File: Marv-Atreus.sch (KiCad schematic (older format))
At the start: 106 parts, among them SW1 SW_Push, U1 ATmega32U4-AU, Y1 16MHz

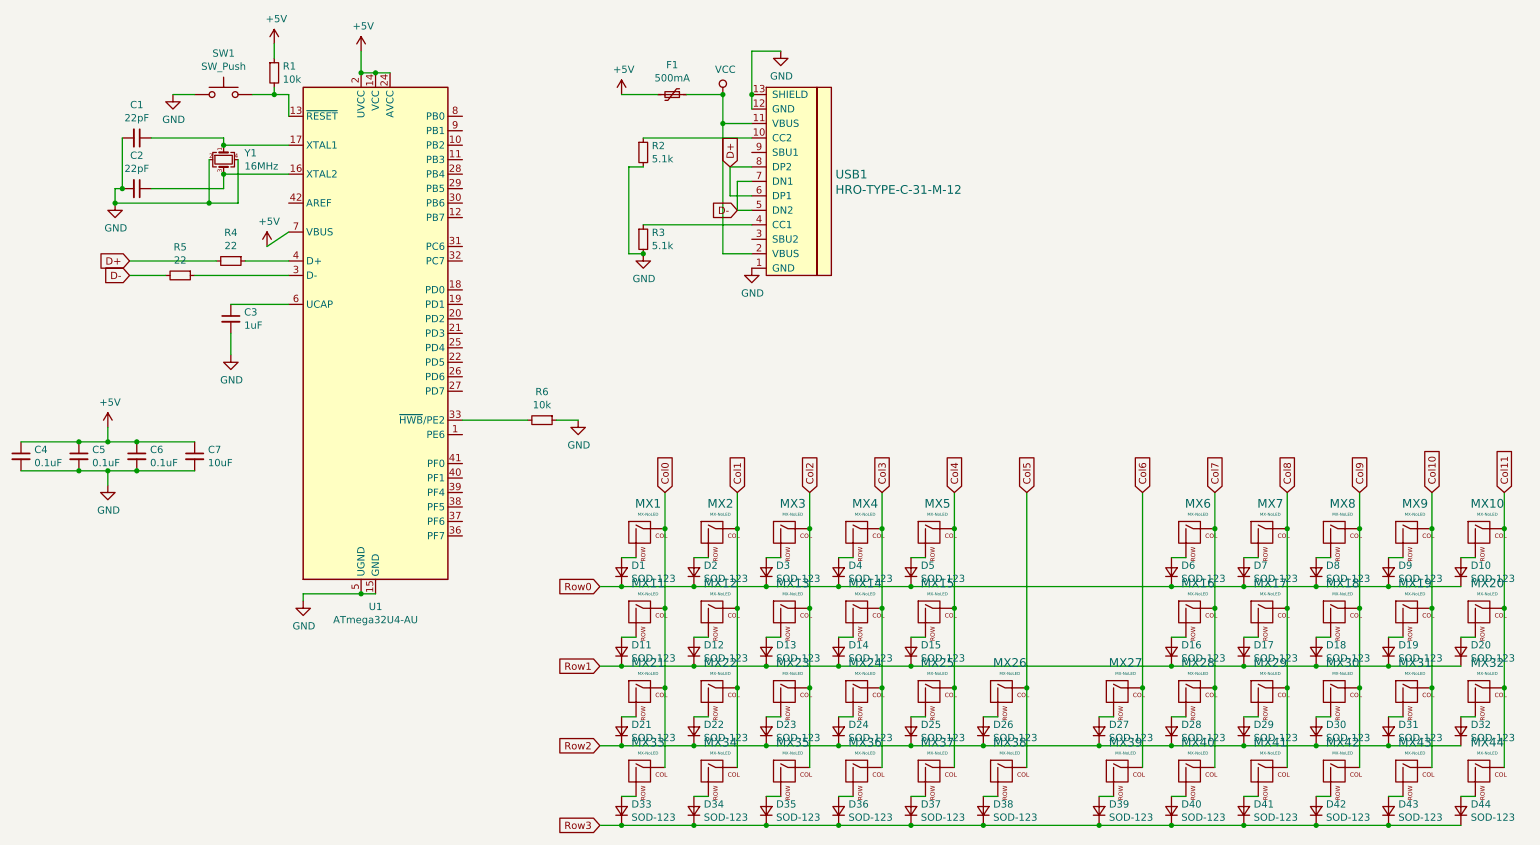
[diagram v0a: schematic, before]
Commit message: First Proto
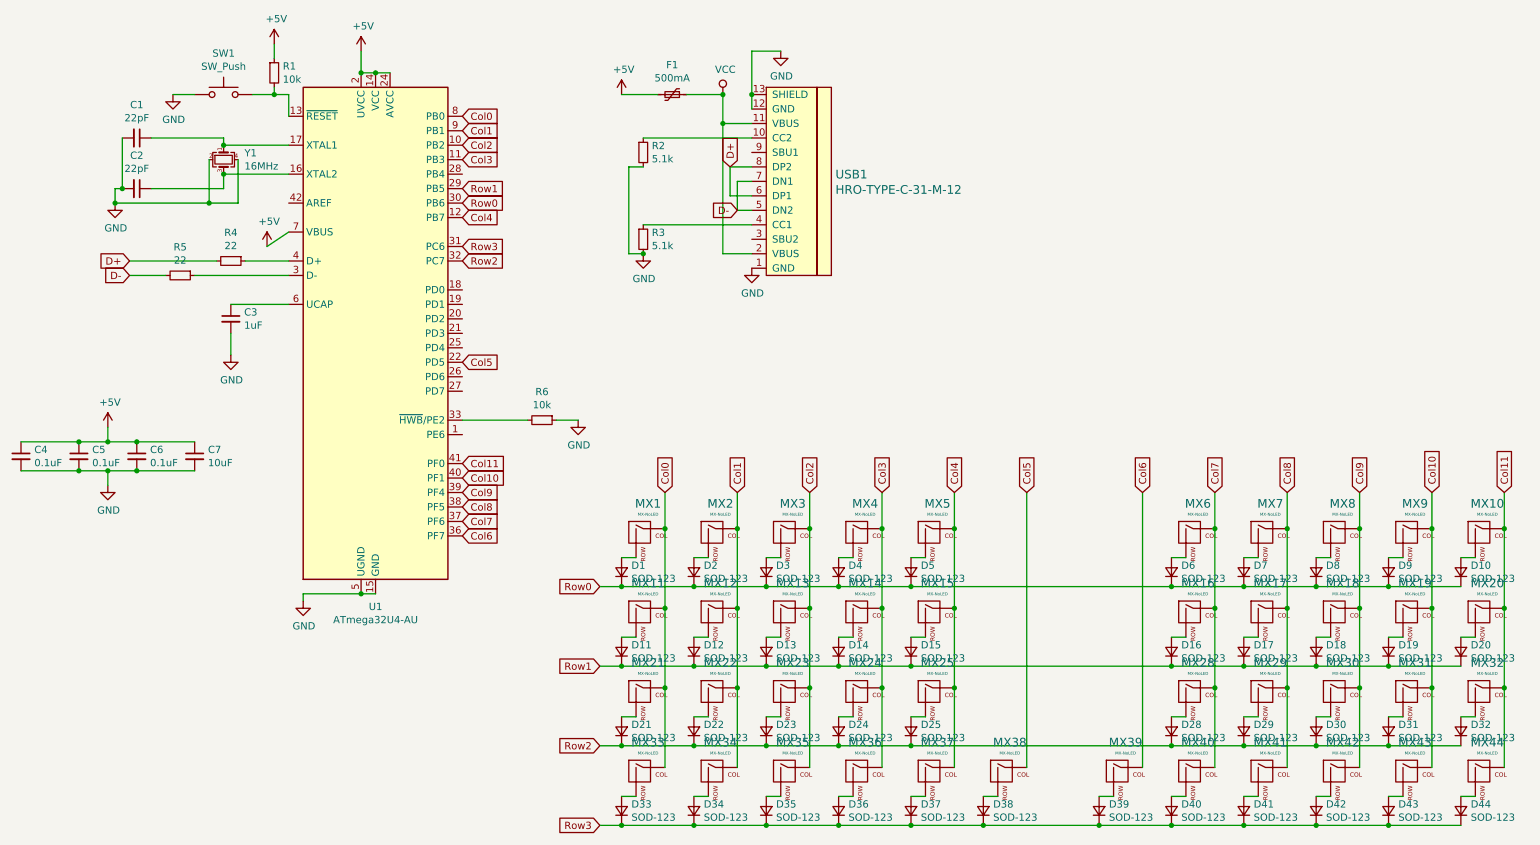
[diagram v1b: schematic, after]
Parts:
- removed D26, D27: SOD-123, Diode_SMD:D_SOD-123, symbol Device:D_Small
- removed MX26, MX27: MX-NoLED, MX_Only:MXOnly-1U-NoLED, symbol MX_Alps_Hybrid:MX-NoLED
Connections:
- net Col0: now also U1.8 (PB0)
- net Col1: now also U1.9 (PB1)
- net Col10: now also U1.40 (PF1)
- net Col11: now also U1.41 (PF0)
- net Col2: now also U1.10 (PB2)
- net Col3: now also U1.11 (PB3)
- net Col4: now also U1.12 (PB7)
- net Col5: now also U1.22 (PD5)
- net Col6: now also U1.36 (PF7)
- net Col7: now also U1.37 (PF6)
- net Col8: now also U1.38 (PF5)
- net Col9: now also U1.39 (PF4)
- net Row0: now also U1.30 (PB6)
- net Row1: now also U1.29 (PB5)
- net Row2: now also U1.32 (PC7)
- net Row3: now also U1.31 (PC6)
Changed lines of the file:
@@
 	6750 5900 6850 5900
-$Comp
-L MX_Alps_Hybrid:MX-NoLED MX26
-U 1 1 5EA47DBA
-P 7400 5200
-F 0 "MX26" H 7433 5423 60  0000 C CNN
-F 1 "MX-NoLED" H 7433 5349 20  0000 C CNN
-F 2 "MX_Only:MXOnly-1U-NoLED" H 6775 5175 60  0001 C CNN
-F 3 "" H 6775 5175 60  0001 C CNN
-	1    7400 5200
-	1    0    0    -1
-$EndComp
-$Comp
-L Device:D_Small D26
-U 1 1 5EA47DC4
-P 7250 5450
-F 0 "D26" V 7296 5382 50  0000 R CNN
-F 1 "SOD-123" V 7205 5382 50  0000 R CNN
-F 2 "Diode_SMD:D_SOD-123" V 7250 5450 50  0001 C CNN
-F 3 "~" V 7250 5450 50  0001 C CNN
-	1    7250 5450
-	0    -1   -1   0
-$EndComp
-Wire Wire Line
-	7250 5350 7350 5350
 $Comp
 L MX_Alps_Hybrid:MX-NoLED MX38
@@
 	8550 5900 8650 5900
 $Comp
-L MX_Alps_Hybrid:MX-NoLED MX27
-U 1 1 5EA954FD
-P 8200 5200
-F 0 "MX27" H 8233 5423 60  0000 C CNN
-F 1 "MX-NoLED" H 8233 5349 20  0000 C CNN
-F 2 "MX_Only:MXOnly-1U-NoLED" H 7575 5175 60  0001 C CNN
-F 3 "" H 7575 5175 60  0001 C CNN
-	1    8200 5200
-	1    0    0    -1
-$EndComp
-$Comp
-L Device:D_Small D27
-U 1 1 5EA95507
-P 8050 5450
-F 0 "D27" V 8096 5382 50  0000 R CNN
-F 1 "SOD-123" V 8005 5382 50  0000 R CNN
-F 2 "Diode_SMD:D_SOD-123" V 8050 5450 50  0001 C CNN
-F 3 "~" V 8050 5450 50  0001 C CNN
-	1    8050 5450
-	0    -1   -1   0
-$EndComp
-Wire Wire Line
-	8050 5350 8150 5350
-$Comp
 L MX_Alps_Hybrid:MX-NoLED MX39
 U 1 1 5EA95512
@@
 Wire Wire Line
 	6750 5550 6250 5550
-Connection ~ 7250 5550
-Wire Wire Line
-	7250 5550 6750 5550
-Connection ~ 8050 5550
-Wire Wire Line
-	8050 5550 7250 5550
 Connection ~ 8550 5550
-Wire Wire Line
-	8550 5550 8050 5550
 Connection ~ 9050 5550
 Wire Wire Line
@@
 Wire Wire Line
 	7050 5150 7050 4600
-Wire Wire Line
-	7550 5700 7550 5150
-Connection ~ 7550 5150
-Wire Wire Line
-	7550 5150 7550 3800
-Wire Wire Line
-	8350 5700 8350 5150
-Connection ~ 8350 5150
-Wire Wire Line
-	8350 5150 8350 3800
 Wire Wire Line
 	8850 5700 8850 5150
@@
 Text GLabel 10850 3800 1    50   Input ~ 0
 Col11
+Wire Wire Line
+	7550 3800 7550 5700
+Wire Wire Line
+	8350 3800 8350 5700
+Wire Wire Line
+	6750 5550 8550 5550
+Text GLabel 3650 4100 2    50   Input ~ 0
+Col6
+Text GLabel 3650 3900 2    50   Input ~ 0
+Col8
+Text GLabel 3650 3800 2    50   Input ~ 0
+Col9
+Text GLabel 3650 3700 2    50   Input ~ 0
+Col10
+Text GLabel 3650 4000 2    50   Input ~ 0
+Col7
+Text GLabel 3650 3600 2    50   Input ~ 0
+Col11
+Text GLabel 3650 1200 2    50   Input ~ 0
+Col0
+Text GLabel 3650 1300 2    50   Input ~ 0
+Col1
+Text GLabel 3650 1400 2    50   Input ~ 0
+Col2
+Text GLabel 3650 1500 2    50   Input ~ 0
+Col3
+Text GLabel 3650 1900 2    50   Input ~ 0
+Col4
+Text GLabel 3650 2900 2    50   Input ~ 0
+Col5
+Text GLabel 3650 1700 2    50   Input ~ 0
+Row1
+Text GLabel 3650 1800 2    50   Input ~ 0
+Row0
+Text GLabel 3650 2100 2    50   Input ~ 0
+Row3
+Text GLabel 3650 2200 2    50   Input ~ 0
+Row2
 $EndSCHEMATC
